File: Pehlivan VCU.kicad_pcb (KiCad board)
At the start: 2 copper layers, 90 x 90 mm, 72 parts, among them J1 PWR_IN, J10 Headlights, J11 Blinker, J12 Stop, J2 DEBUG, J3 Nextion, J4 CAN, J5 SD_CARD MODULE, J6 LORA, J7 IN1, J8 IN2, J9 GND, Q4 BC817, Q5 BC817, U1 L7805, U10 STM32G431C8Tx, U2 LM1117MP-3.3, U3 TJA1051T-3, U5 BTS432, U6 BTS432, U7 BTS432, U8 BTS432, U9 BTS432, Y2 16MHz 18pF

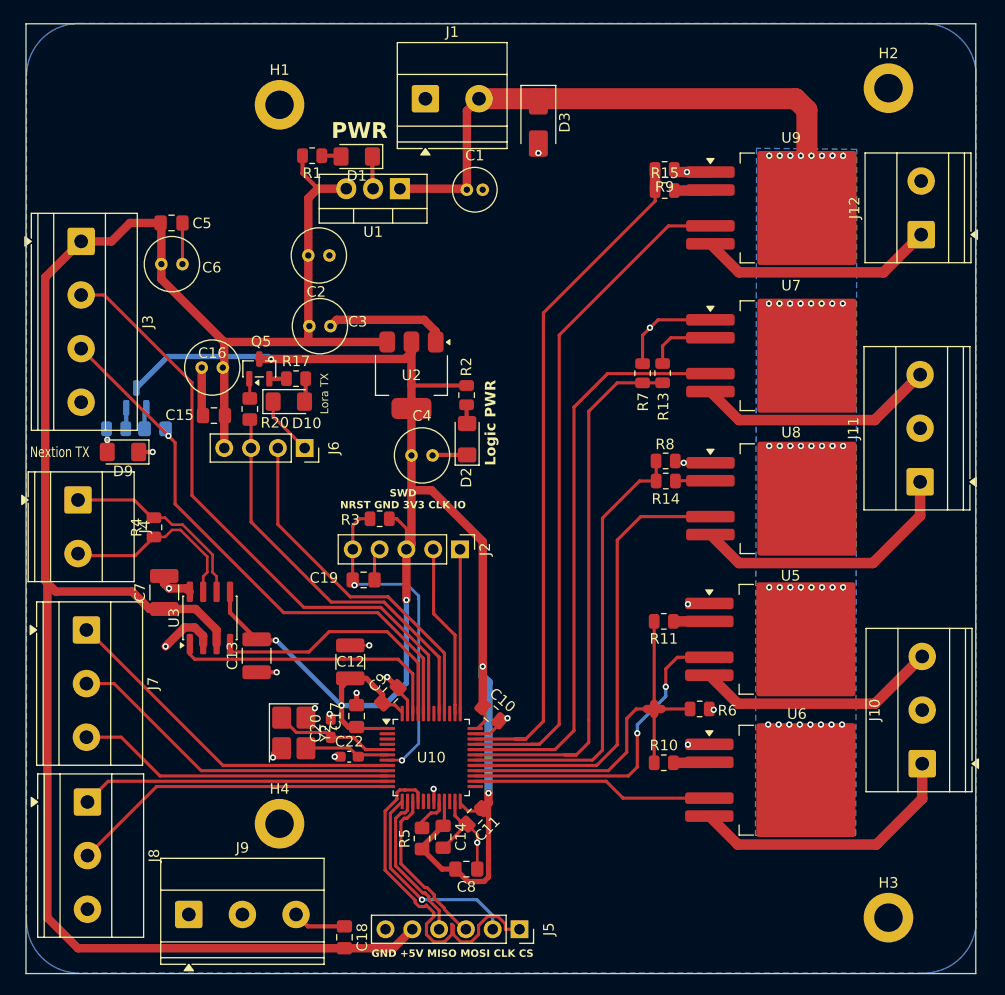
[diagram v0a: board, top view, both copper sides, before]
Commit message: changes
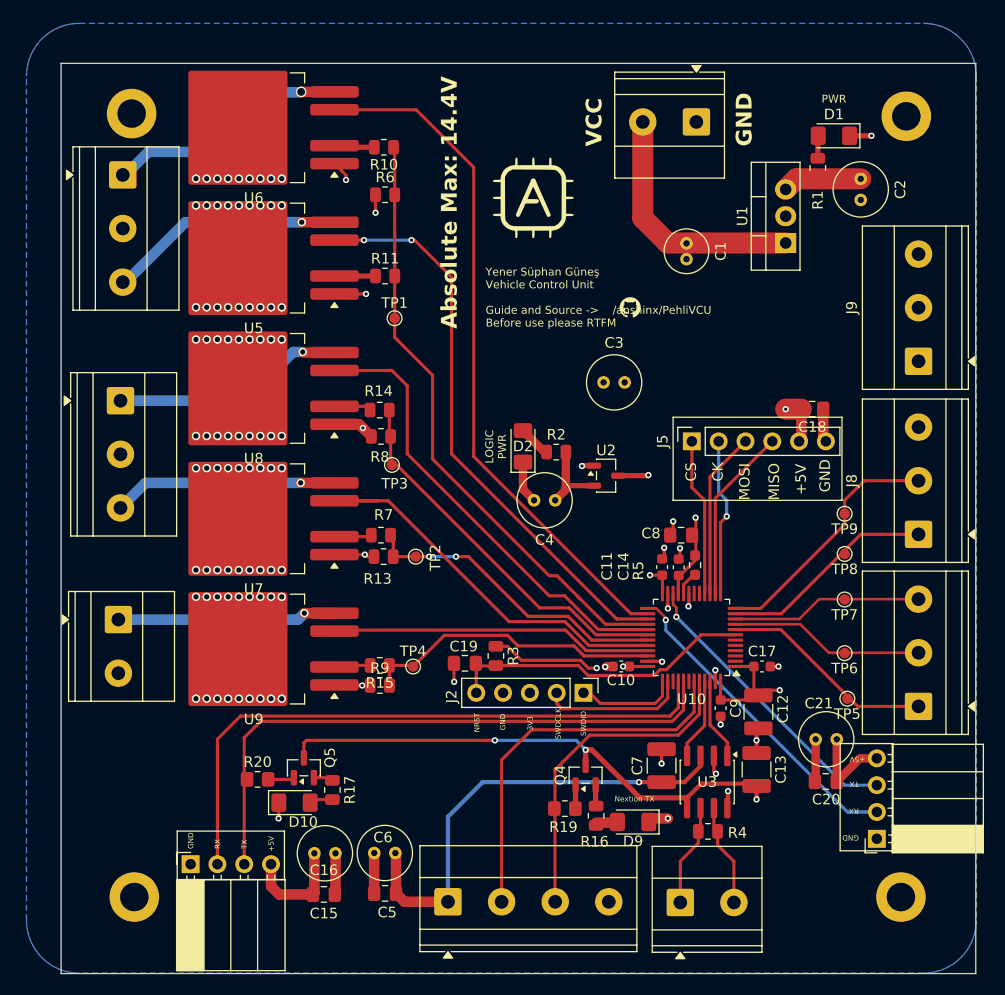
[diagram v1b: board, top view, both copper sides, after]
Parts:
- removed C22: 26pF, Capacitor_SMD:C_0603_1608Metric_Pad1.08x0.95mm_HandSolder
- removed D3: SMAJ16CA, Diode_SMD:D_SMA
- removed Y2: 16MHz 18pF, Crystal:Crystal_SMD_3225-4Pin_3.2x2.5mm_HandSoldering
- added C21: 10uF, Capacitor_THT:C_Radial_D5.0mm_H5.0mm_P2.00mm, F.Cu at (180.1, 127.8)
- added G***: LOGO, LOGO, F.Cu at (151.1, 76.3)
- added G***: LOGO, LOGO, F.Cu at (160.5, 86.9)
- added G***: LOGO, LOGO, B.Cu at (143.2, 69.1)
- added G***: LOGO, LOGO, B.Cu at (151.7, 76.3)
- added J13: LORA, Connector_PinSocket_2.54mm:PinSocket_1x04_P2.54mm_Horizontal, F.Cu at (183.9, 137.2)
- added TP1: TestPoint, TestPoint:TestPoint_Pad_D1.0mm, F.Cu at (138.2, 87.9)
- added TP2: TestPoint, TestPoint:TestPoint_Pad_D1.0mm, F.Cu at (140.2, 110.5)
- added TP3: TestPoint, TestPoint:TestPoint_Pad_D1.0mm, F.Cu at (137.9, 101.8)
- added TP4: TestPoint, TestPoint:TestPoint_Pad_D1.0mm, F.Cu at (140.0, 120.9)
- added TP5: TestPoint, TestPoint:TestPoint_Pad_D1.0mm, F.Cu at (181.1, 124.0)
- added TP6: TestPoint, TestPoint:TestPoint_Pad_D1.0mm, F.Cu at (180.8, 119.6)
- added TP7: TestPoint, TestPoint:TestPoint_Pad_D1.0mm, F.Cu at (180.8, 114.6)
- added TP8: TestPoint, TestPoint:TestPoint_Pad_D1.0mm, F.Cu at (180.8, 110.2)
- added TP9: TestPoint, TestPoint:TestPoint_Pad_D1.0mm, F.Cu at (180.8, 106.4)
- C10, C11, C14, C17, C9: footprint Capacitor_SMD:C_0805_2012Metric_Pad1.18x1.45mm_HandSolder -> Capacitor_SMD:C_0603_1608Metric
- C20: value 26pF -> 100nF; footprint Capacitor_SMD:C_0603_1608Metric_Pad1.08x0.95mm_HandSolder -> Capacitor_SMD:C_0805_2012Metric_Pad1.18x1.45mm_HandSolder
- J6: footprint Connector_PinSocket_2.54mm:PinSocket_1x04_P2.54mm_Vertical -> Connector_PinSocket_2.54mm:PinSocket_1x04_P2.54mm_Horizontal
- Q4, R16, R19: moved to F.Cu
- R5: footprint Resistor_SMD:R_0805_2012Metric_Pad1.20x1.40mm_HandSolder -> Resistor_SMD:R_0603_1608Metric_Pad0.98x0.95mm_HandSolder
- U2: value LM1117MP-3.3 -> XC6206P332MR; footprint Package_TO_SOT_SMD:SOT-223-3_TabPin2 -> Package_TO_SOT_SMD:SOT-23-3
- moved J10 94.1 mm to (112.4, 74.3), turned to -90 degrees
- moved J9 86.8 mm to (187.8, 92.0), turned to 90 degrees
- moved J12 84.4 mm to (112.0, 116.5), turned to -90 degrees
- moved J8 82.7 mm to (187.8, 108.4), turned to 90 degrees
- moved U6 80.0 mm to (124.8, 69.8), turned to 180 degrees
- moved J7 79.2 mm to (187.8, 124.7), turned to 90 degrees
- moved J11 76.2 mm to (112.2, 95.7), turned to -90 degrees
- moved H2 71.8 mm to (113.3, 68.5)
- moved J3 71.6 mm to (143.3, 143.2), turned to 0 degrees
- moved H3 71.5 mm to (113.5, 142.7)
- moved J4 68.6 mm to (165.3, 143.3), turned to 0 degrees
- moved C18 66.9 mm to (177.8, 96.5), turned to 180 degrees
- moved C5 66.7 mm to (137.3, 142.4), turned to 0 degrees
- moved U9 65.9 mm to (124.8, 119.2), turned to 180 degrees
- moved R10 64.1 mm to (137.2, 71.7), turned to 180 degrees
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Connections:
- C20 pad 1: /HSE_IN -> GND
- C20 pad 2: GND -> +5V
- U10 pad 22: unconnected-(U10-PB10-Pad22) -> /UART3_TX
- U10 pad 25: unconnected-(U10-PB11-Pad25) -> /UART3_RX
- U10 pad 5: /HSE_IN -> unconnected-(U10-PF0-Pad5)
- U10 pad 6: /HSE_OUT -> unconnected-(U10-PF1-Pad6)
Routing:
- net +5V: track 190.2 -> 78.1 mm, vias 0 -> 3
- net +3V3: track 174.7 -> 95.8 mm, vias 6 -> 8
- net /L_HL_FAULT: track 22.9 -> 65.5 mm
- net /F_BrakeLights: track 64.9 -> 28.4 mm
- net /Brake_FAULT: track 65.1 -> 30.5 mm
- net VCC: track 56.3 -> 23.6 mm, vias 40 -> 81
- net /UART3_RX: track 0.00 -> 30.4 mm, vias 0 -> 1
- net /UART3_TX: track 0.00 -> 27.9 mm, vias 0 -> 1
- net GND: track 92.1 -> 64.5 mm, vias 21 -> 25
- net /UART2_RX: track 33.8 -> 59.2 mm
- net /R_HL_FAULT: track 30.7 -> 54.4 mm
- net /UART1_RX: track 59.4 -> 36.5 mm
- net /L_Blinker: track 51.9 -> 29.5 mm, vias 0 -> 2
- net /UART1_TX: track 53.2 -> 31.5 mm, vias 1 -> 0
- net /UART2_TX: track 38.2 -> 57.4 mm
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- added copper zone on In2.Cu, net +3V3
- added copper zone on In2.Cu, net +5V
- added copper zone on In1.Cu, net GND
- added copper zone on In2.Cu, net VCC
- removed copper zone on B.Cu, net VCC
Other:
- board size 90 x 90 mm -> 86.7 x 86.2 mm
- copper layers 2 -> 4
- board text added: "+5V"
- board text added: "3V3"
- board text added: "Absolute Max: 14.4V"
- board text added: "BRAKE"
- board text added: "Blinkers"
- board text added: "CANBUS"
- board text added: "CK"
- board text added: "CS"
- board text added: "Hazards"
- board text added: "Headlight"
- board text added: "High"
- board text added: "LOGIC PWR"
- board text added: "Left"
- board text added: "Left Signal"
- board text added: "Low"
- board text added: "MISO"
- board text added: "MOSI"
- board text added: "NRST"
- board text added: "NXVCU Rev.02"
- board text added: "Output"
- board text added: "Right"
- board text added: "Right Signal"
- board text added: "SWDCLK"
- board text added: "SWDIO"
- board text added: "Stop Light"
- board text added: "UART (GPS)"
- board text added: "UART (Lora)"
- board text added: "UART (Nextion)"
- board text added: "VCC"
- board text added: "Yener Süphan Güneş Vehicle Control Unit Guide and Source -> /anshinx/PehliVCU Before use please RTFM"
- board text removed: "5V"
- board text removed: "Brake IN"
- board text removed: "CAN"
- board text removed: "GND +5V MISO MOSI CLK CS"
- board text removed: "H"
- board text removed: "Hazards In"
- board text removed: "L"
- board text removed: "Left Blinker"
- board text removed: "Left Headlight"
- board text removed: "Left Signal In"
- board text removed: "Logic PWR"
- board text removed: "Lora TX"
- board text removed: "Nextion Output"
- board text removed: "Right Blinker"
- board text removed: "Right Headlight"
- board text removed: "Right Signal In"
- board text removed: "SWD NRST GND 3V3 CLK IO"
- board text removed: "Stop"
